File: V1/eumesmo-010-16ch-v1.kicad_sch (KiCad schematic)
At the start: 8 parts, among them J1 250-208, J2 250-208, J3 250-208, J4 250-208

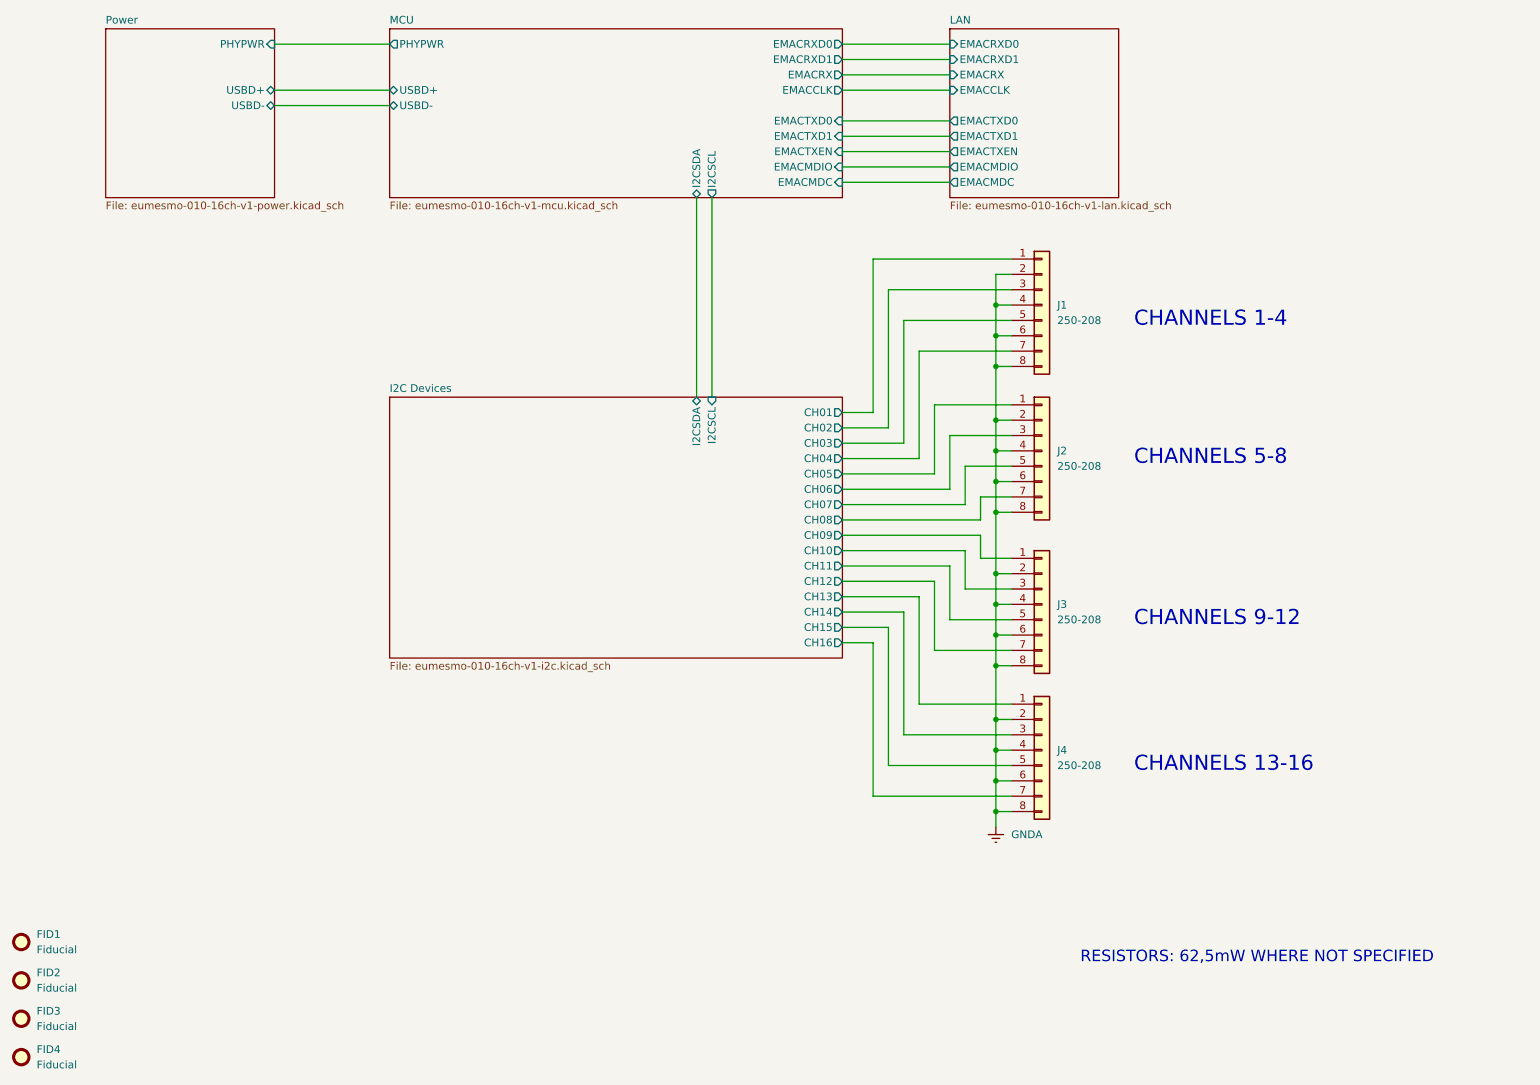
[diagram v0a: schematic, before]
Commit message: Development
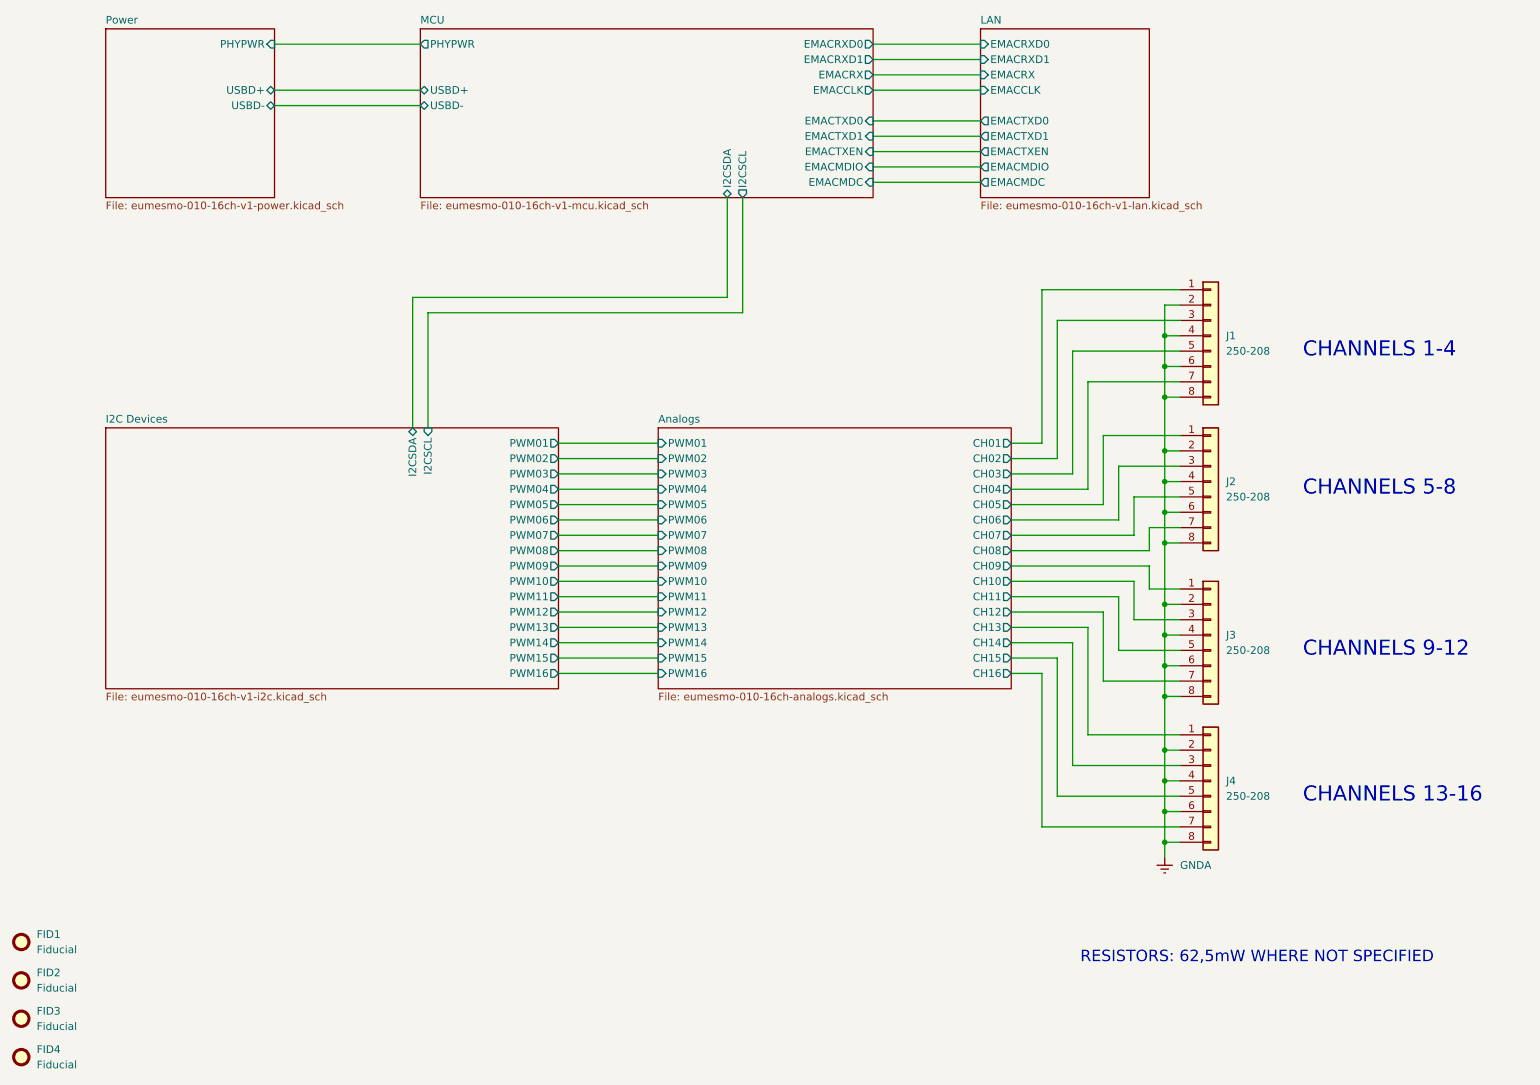
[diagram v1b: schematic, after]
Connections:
- net I2C Devices/CH01 renamed Analogs/CH01
- net I2C Devices/CH02 renamed Analogs/CH02
- net I2C Devices/CH03 renamed Analogs/CH03
- net I2C Devices/CH04 renamed Analogs/CH04
- net I2C Devices/CH05 renamed Analogs/CH05
- net I2C Devices/CH06 renamed Analogs/CH06
- net I2C Devices/CH07 renamed Analogs/CH07
- net I2C Devices/CH08 renamed Analogs/CH08
- net I2C Devices/CH09 renamed Analogs/CH09
- net I2C Devices/CH10 renamed Analogs/CH10
- net I2C Devices/CH11 renamed Analogs/CH11
- net I2C Devices/CH12 renamed Analogs/CH12
- net I2C Devices/CH13 renamed Analogs/CH13
- net I2C Devices/CH14 renamed Analogs/CH14
- net I2C Devices/CH15 renamed Analogs/CH15
- net I2C Devices/CH16 renamed Analogs/CH16
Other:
- added sheet Analogs (eumesmo-010-16ch-analogs.kicad_sch)
- sheet I2C Devices ports: added PWM01, PWM02, PWM03, PWM04, PWM05, PWM06, PWM07, PWM08, PWM09, PWM10, PWM11, PWM12, PWM13, PWM14, PWM15, PWM16; removed CH01, CH02, CH03, CH04, CH05, CH06, CH07, CH08, CH09, CH10, CH11, CH12, CH13, CH14, CH15, CH16
- moved on the sheet: J1, J2, J3, J4

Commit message: Development
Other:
- title: eumesmo 24V 16xIn/16xOut/1-Wire Module -> eumesmo 24V 16x 0-10V module
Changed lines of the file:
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@@
 	(paper "A4")
 	(title_block
-		(title "eumesmo 24V 16xIn/16xOut/1-Wire Module")
-		(date "2026-06-17")
-		(rev "V6.2")
+		(title "eumesmo 24V 16x 0-10V module")
+		(date "2026-06-23")
+		(rev "V1.0")
 	)
 	(text "CHANNELS 9-12"
